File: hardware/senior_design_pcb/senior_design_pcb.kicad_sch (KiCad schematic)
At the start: 90 parts, among them J1 SBH11-PBPC-D05-ST-BK, J10 Conn_01x04_Socket, J11 2x08Rectangle-LED Matrix Conn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, J12 1x05JST - Joystick2 connector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, J13 UJ20-C-H-C-4-SMT-TR, J2 Conn_01x08_Pin, J3 Conn_01x02_Socket, J4 Conn_01x02_Socket, J5 1x05JST-Admin LCD Console Con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, J6 1x05JST - Joystick1 connector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, J9 Conn_01x04_Socket, SW3 1x02JST-Admin Console button 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, U1 KMR241GLFS, U10 KMR241GLFS, U2 STM32F091RCTx, U3 LD1117S33TR_SOT223, U4 KMR241GLFS, U5 USBLC6-2SC6Y, U6 2SA1873-GRTE85L_F, U7 2SA1873-GRTE85L_F, U8 2SA1873-GRTE85L_F, U9 KMR241GLFS

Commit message: cleaned up
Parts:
- removed TP1: TestPoint_Small, TestPoint:TestPoint_Pad_D1.5mm, symbol Connector:TestPoint_Small
- C20, C21: value 12.5pF -> 15pF
- FT1: value ~ -> FT232
- J1: footprint General Library:jtag_conn -> Sr_ Design:jtag_conn
- U1, U10, U4, U9: footprint General Library:KMR241G-RESET-BUTTON -> kicad_library:KMR241G-RESET-BUTTON
- U5: footprint kicad_library:TVS-DIODE-USBLC6-2SC6Y -> Sr_ Design:TVS-DIODE-USBLC6-2SC6Y
- XTAL2: value 8MHz(8PF) -> 8MHz(15pF)
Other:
- note added: "mounting holes"
- note removed: "600 Ohm @ 100MHz .3 Ohm DCR, 500 mA"
- note removed: "BOOT0 PDR"
- note removed: "Communications"
- note removed: "one for each pin connected to VDD, 4.7uF bulk caps near source"
- note removed: "should we have a clock select jumper like the 362 board?"
- note removed: "two diff kinds of tp - pad (left) and drill hole (right):"
- moved on the sheet: C1, C10, C11, C12, C13, C14, C15, C16, C17, C18, C19, C2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

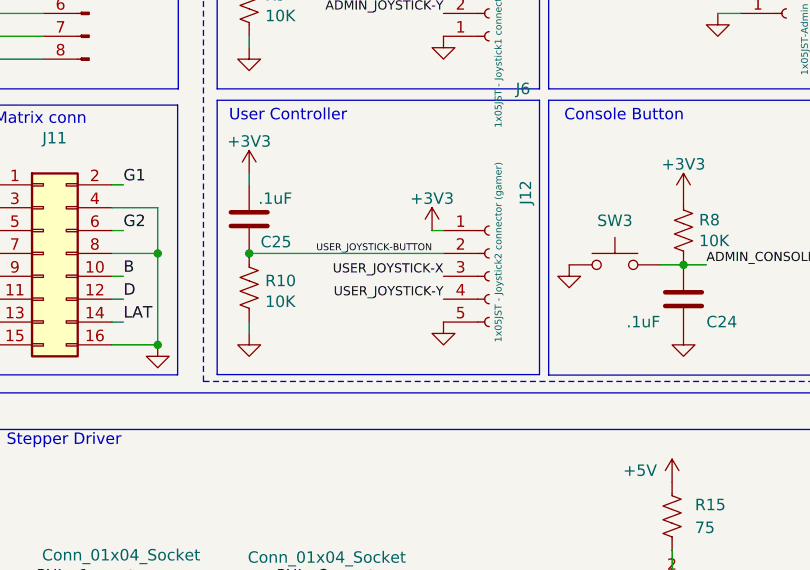
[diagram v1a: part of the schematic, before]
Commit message: reorganized
updated + finished reorg
added footprints
added 2x8 jtag 3d file
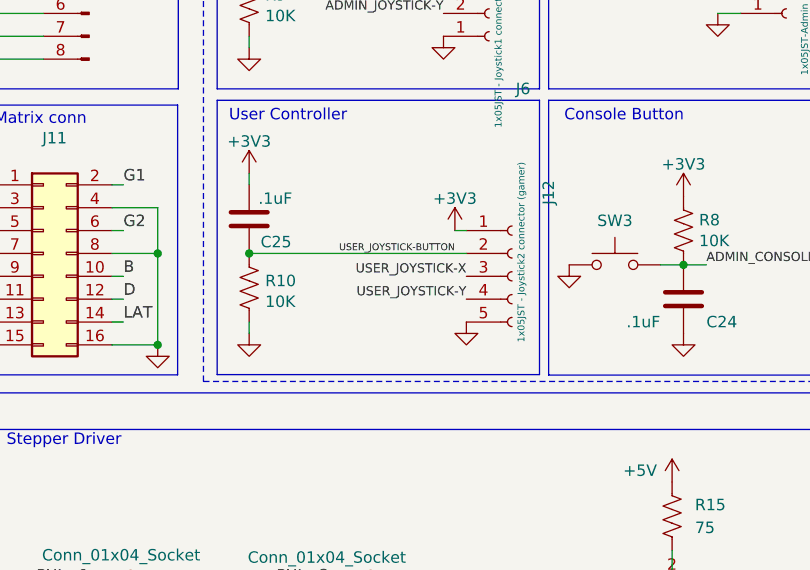
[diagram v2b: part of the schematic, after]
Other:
- moved on the sheet: J12
